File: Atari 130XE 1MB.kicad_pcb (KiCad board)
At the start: 2 copper layers, 324 x 204 mm, 349 parts, among them J1 SIO, J10 Mem_on_off, J100 cond, J101 cond, J102 pin, J103 pin, J104 pin, J105 pin, J106 pin, J107 pin, J108 pin, J109 pin, J110 pin, J111 pin, J2 Video, J201 Diagnostic, J202 Diag, J210 Diag, J211 Diag, J212 Diag, J24 Cartridge, J4 Expansion, J5 Joystick_Port, J6 Joystick_Port, J7 Power, J8 Keyboard, M1 Modulator, Q1 2N3904, Q2 2N3904, Q3 2N3904, Q4 2N3906, Q6 2N3904, SW1 Switch_power_on, U1 LM358, U10 DRAM_4464, U17 GTIA, U18 74LS08, U19 LM555, U2 74LS138, U20 4050, U21 74LS74, U22 POKEY, U23 PIA, U24 CD4051B, U25 CD4051B, U3 MMU, U4 BASIC_ROM, U40 GAL20V8_DIP, U41 74LS157, U42 74LS175, U43 DRAM_1MB_4bit, U44 DRAM_1MB_4bit, U5 27C128, U6 Freddie, U7 Antic, U8 Sally, U9 DRAM_4464, Y1 Crystal, Y2 4,43 MHz

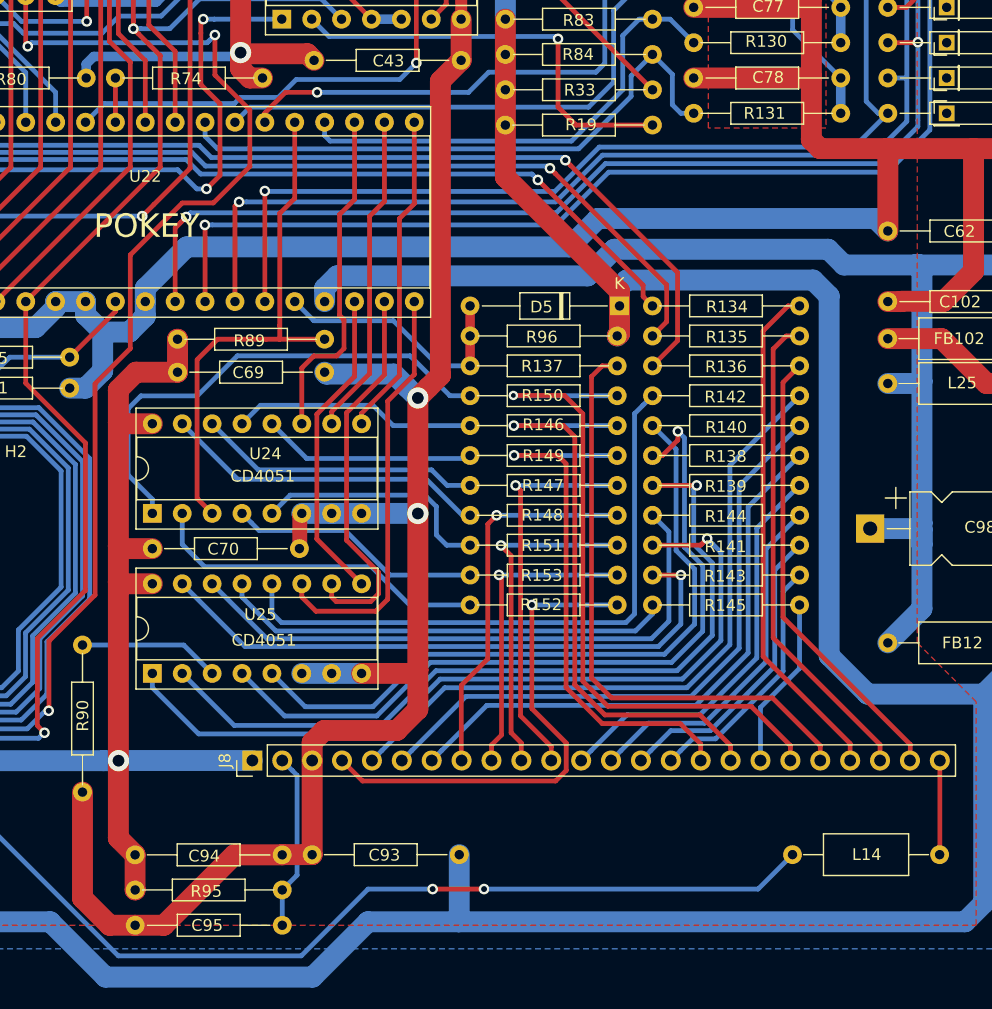
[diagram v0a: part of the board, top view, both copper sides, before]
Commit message: Tracking
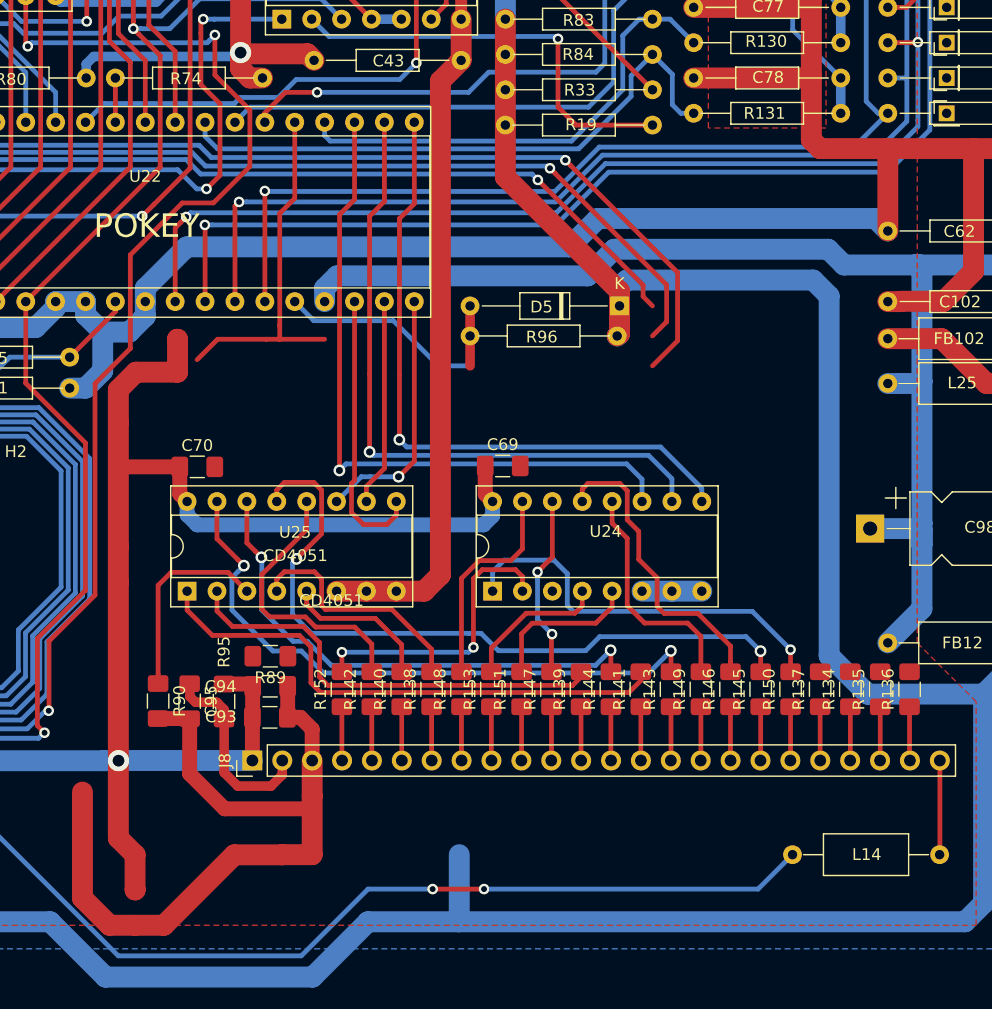
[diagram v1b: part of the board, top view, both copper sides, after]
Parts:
- C69, C70, C93, C94, C95: footprint Atari:C_Axial_L5.1mm_D2.5mm_P12.50mm_Horizontal -> Capacitor_SMD:C_1206_3216Metric_Pad1.42x1.75mm_HandSolder
- R134, R135, R136, R137, R138, R139, R140, R141, R142, R143, R144, R145, R146, R147, R148, R149, R150, R151, R152, R153, R89, R90, R95: footprint Atari:R_Axial_DIN0207_L3.6mm_D2.2mm_P10.16mm_Horizontal -> Resistor_SMD:R_1206_3216Metric_Pad1.42x1.75mm_HandSolder
- moved R142 44.1 mm to (294.5, 202.8), turned to 90 degrees
- moved R140 40.6 mm to (297.1, 202.8), turned to 90 degrees
- moved R138 37.0 mm to (299.6, 202.8), turned to 90 degrees
- moved R134 32.9 mm to (335.2, 202.8), turned to 90 degrees
- moved R137 32.4 mm to (332.6, 202.8), turned to 90 degrees
- moved R135 30.8 mm to (337.7, 202.8), turned to 90 degrees
- moved U24 29.7 mm to (304.8, 194.5)
- moved R136 29.0 mm to (340.2, 202.8), turned to 90 degrees
- moved R150 29.0 mm to (330.1, 202.8), turned to 90 degrees
- moved C69 28.8 mm to (305.7, 183.8)
- moved R89 27.3 mm to (285.9, 200.0)
- moved R139 25.4 mm to (312.3, 202.8), turned to 90 degrees
- moved R152 24.5 mm to (292.0, 202.8), turned to 90 degrees
- moved R146 24.4 mm to (325.0, 202.8), turned to 90 degrees
- moved R144 21.8 mm to (314.9, 202.8), turned to 90 degrees
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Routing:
- net IN4: track 59.3 -> 4.58 mm, vias 1 -> 0
- net OUT3: track 58.1 -> 4.57 mm
- net OUT5: track 53.7 -> 4.57 mm
- net IN0: track 52.1 -> 4.57 mm, vias 1 -> 0
- net BSC: track 51.2 -> 4.57 mm
- net Net-(R140-Pad2): track 58.4 -> 12.9 mm
- net OUT7: track 49.3 -> 4.57 mm
- net Net-(R138-Pad2): track 64.9 -> 20.4 mm, vias 1 -> 0
- net IN3: track 47.3 -> 4.58 mm, vias 1 -> 0
- net +5VA: track 1975.7 -> 2016.4 mm
- net START: track 43.6 -> 4.58 mm
- net IN6: track 42.7 -> 4.57 mm, vias 1 -> 0
- net SELECT: track 41.4 -> 4.58 mm
- net OPTION: track 38.6 -> 4.58 mm
- net OUT6: track 34.7 -> 4.57 mm
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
